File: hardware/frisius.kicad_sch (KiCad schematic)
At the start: 0 parts

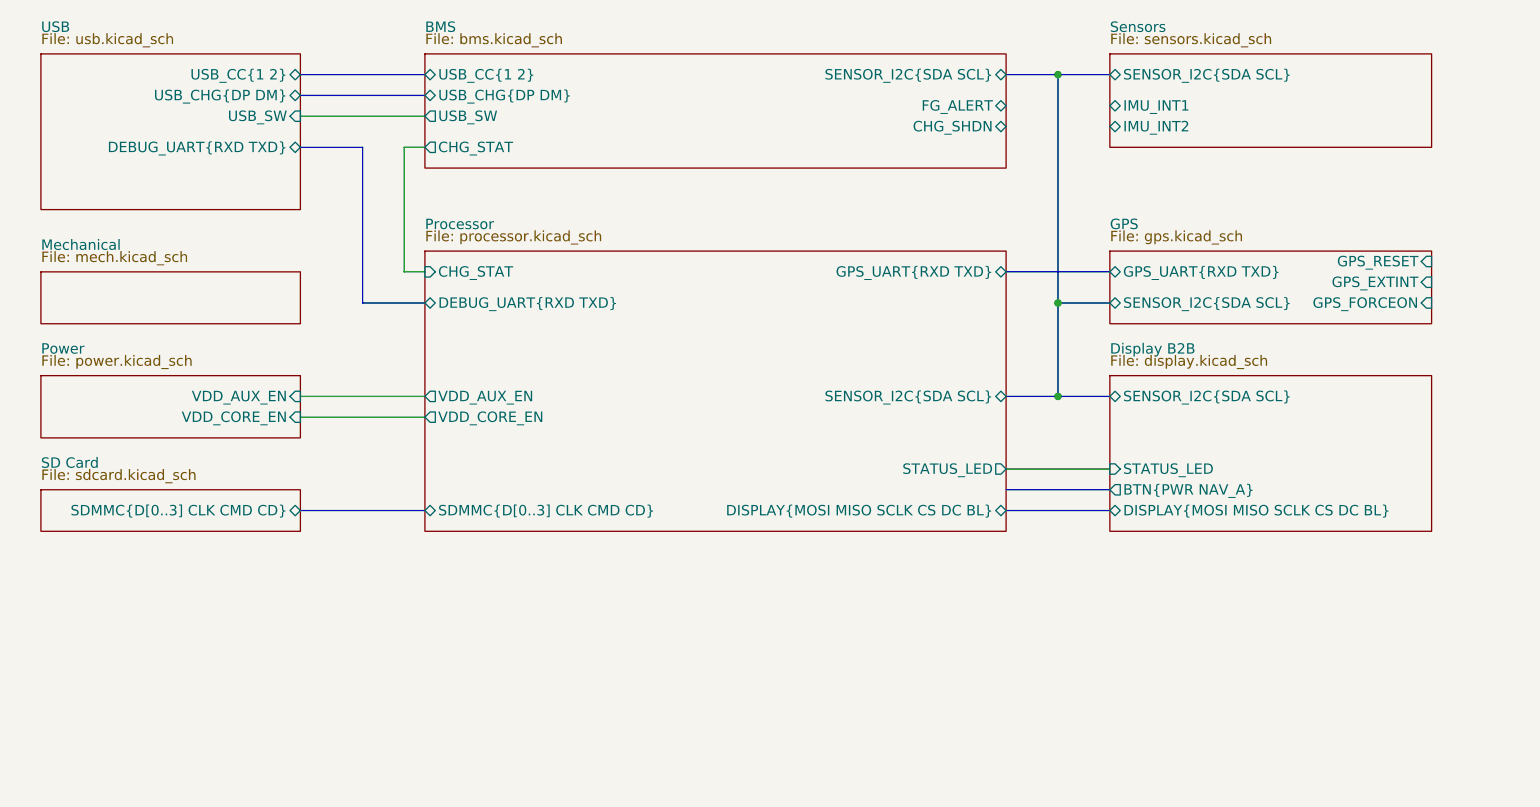
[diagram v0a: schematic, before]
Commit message: started b2b and power
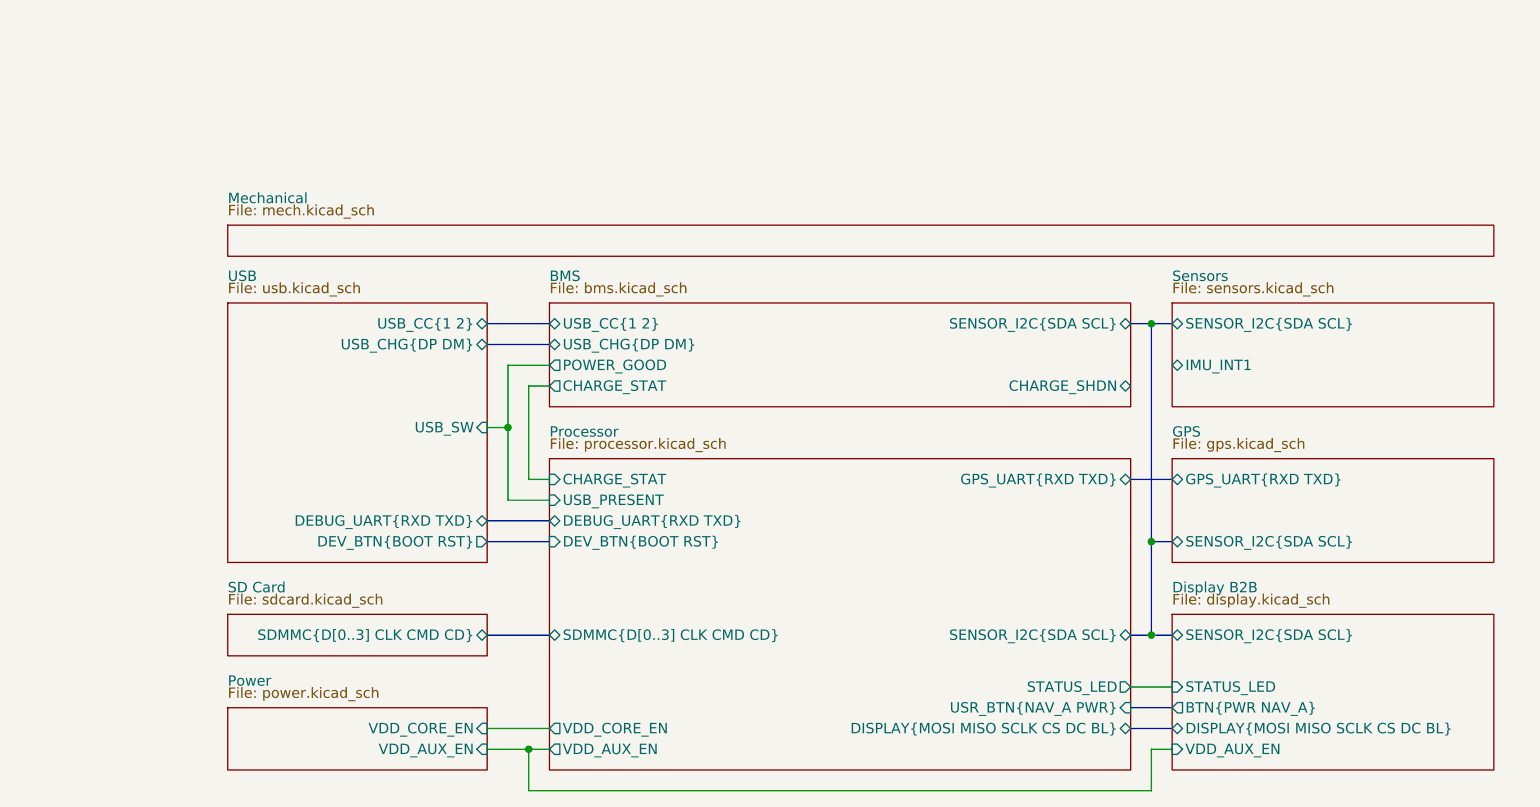
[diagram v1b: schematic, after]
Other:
- sheet BMS ports: added CHARGE_SHDN, CHARGE_STAT, POWER_GOOD; removed CHG_SHDN, CHG_STAT, FG_ALERT, USB_SW
- sheet Display B2B ports: added VDD_AUX_EN; removed none
- sheet GPS ports: added none; removed GPS_EXTINT, GPS_FORCEON, GPS_RESET
- sheet Processor ports: added CHARGE_STAT, DEV_BTN{BOOT RST}, USB_PRESENT, USR_BTN{NAV_A PWR}; removed CHG_STAT
- sheet Sensors ports: added none; removed IMU_INT2
- sheet USB ports: added DEV_BTN{BOOT RST}; removed none
